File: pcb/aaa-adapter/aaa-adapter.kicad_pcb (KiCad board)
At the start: 2 copper layers, 51.5 x 38 mm, 2 parts

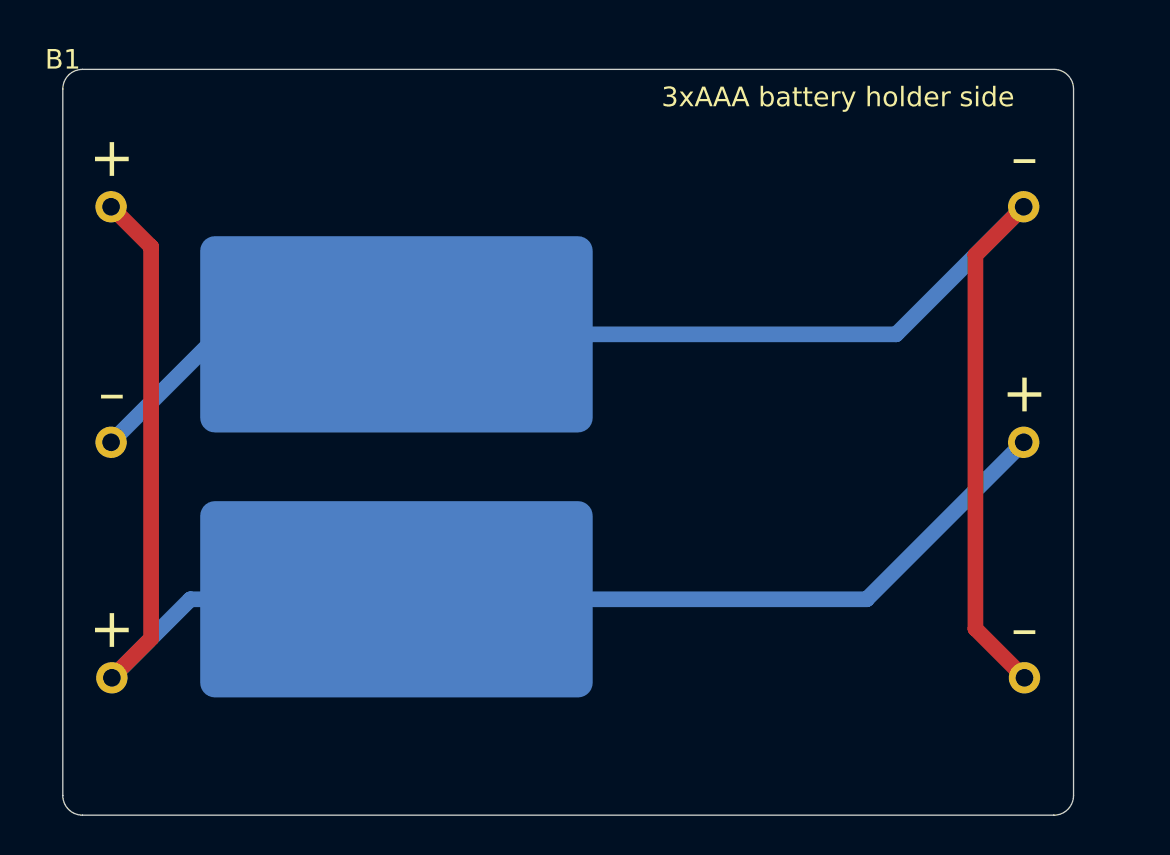
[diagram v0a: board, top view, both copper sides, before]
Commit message: production
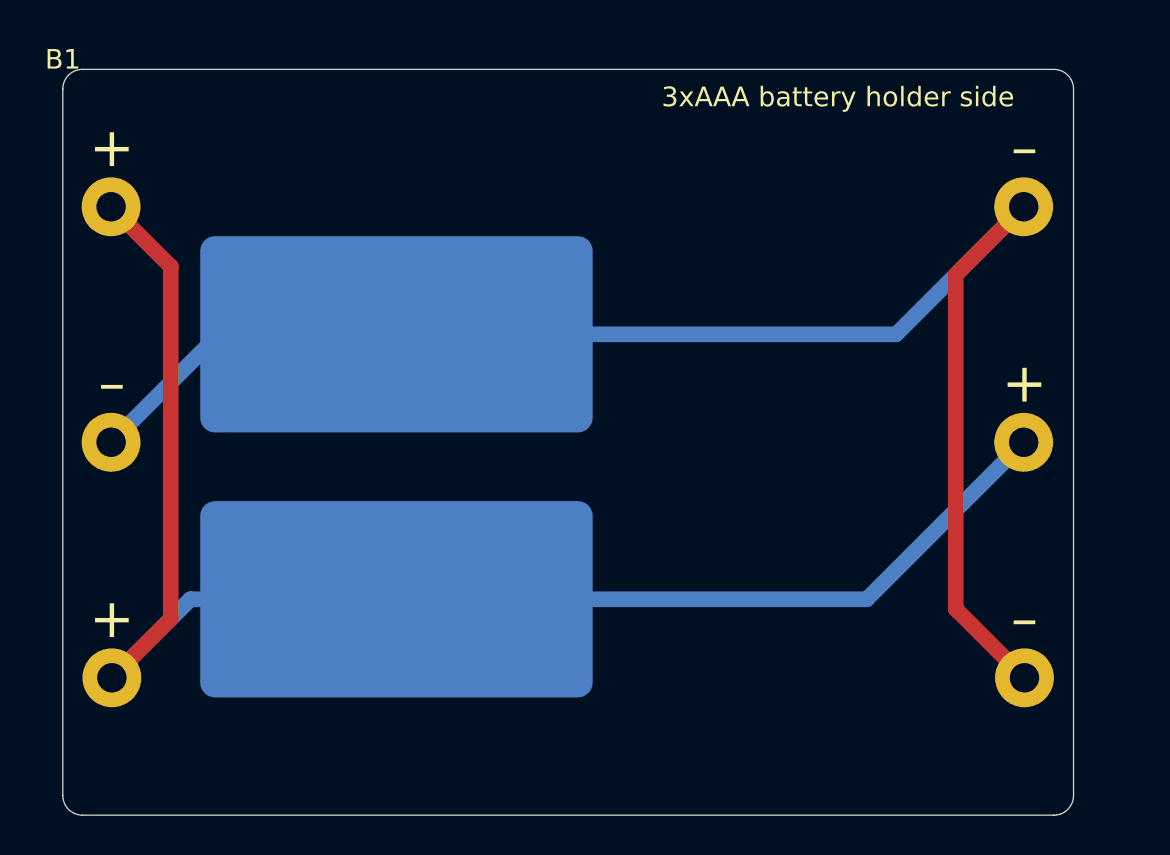
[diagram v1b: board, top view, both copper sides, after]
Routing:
- net /V-: track 77.5 -> 78.4 mm
- net /V+: track 77.1 -> 77.9 mm
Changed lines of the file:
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@@
 		(pad "1" thru_hole circle
 			(at 2.46 7)
-			(size 1.6 1.6)
-			(drill 0.9)
+			(size 3 3)
+			(drill 1.5)
 			(layers "*.Cu" "*.Mask")
 			(remove_unused_layers no)
@@
 		(pad "2" thru_hole circle
 			(at 2.46 19)
-			(size 1.6 1.6)
-			(drill 0.9)
+			(size 3 3)
+			(drill 1.5)
 			(layers "*.Cu" "*.Mask")
 			(remove_unused_layers no)
@@
 		(pad "3" thru_hole circle
 			(at 2.5 31)
-			(size 1.6 1.6)
-			(drill 0.9)
+			(size 3 3)
+			(drill 1.5)
 			(layers "*.Cu" "*.Mask")
 			(remove_unused_layers no)
@@
 		(pad "4" thru_hole circle
 			(at 49 31)
-			(size 1.6 1.6)
-			(drill 0.9)
+			(size 3 3)
+			(drill 1.5)
 			(layers "*.Cu" "*.Mask")
 			(remove_unused_layers no)
@@
 		(pad "5" thru_hole circle
 			(at 48.96 19)
-			(size 1.6 1.6)
-			(drill 0.9)
+			(size 3 3)
+			(drill 1.5)
 			(layers "*.Cu" "*.Mask")
 			(remove_unused_layers no)
@@
 		(pad "6" thru_hole circle
 			(at 48.96 7)
-			(size 1.6 1.6)
-			(drill 0.9)
+			(size 3 3)
+			(drill 1.5)
 			(layers "*.Cu" "*.Mask")
 			(remove_unused_layers no)
@@
 	)
 	(gr_text "–"
-		(at 17.5 31.5 0)
+		(at 17.5 31 0)
 		(layer "F.SilkS")
 		(effects
@@
 	)
 	(gr_text "–"
-		(at 64 19.5 0)
+		(at 64 19 0)
 		(layer "F.SilkS")
 		(effects
@@
 	)
 	(gr_text "+"
-		(at 64 31.5 0)
+		(at 64 31 0)
 		(layer "F.SilkS")
 		(effects
@@
 	)
 	(gr_text "+"
-		(at 17.5 19.5 0)
+		(at 17.5 19 0)
 		(layer "F.SilkS")
 		(effects
@@
 	)
 	(gr_text "+"
-		(at 17.5 43.5 0)
+		(at 17.5 43 0)
 		(layer "F.SilkS")
 		(effects
@@
 	)
 	(gr_text "–"
-		(at 64 43.5 0)
-		(layer "F.SilkS")
-		(effects
-			(font
-				(size 2 2)
-				(thickness 0.25)
-			)
-		)
-	)
-	(segment
-		(start 61.5 43.5)
+		(at 64 43 0)
+		(layer "F.SilkS")
+		(effects
+			(font
+				(size 2 2)
+				(thickness 0.25)
+			)
+		)
+	)
+	(segment
+		(start 60.5 42.5)
 		(end 64 46)
 		(width 0.8)
@@
 	)
 	(segment
-		(start 61.5 24.46)
-		(end 61.5 43.5)
+		(start 63.96 22)
+		(end 60.5 25.46)
 		(width 0.8)
 		(layer "F.Cu")
@@
 	)
 	(segment
-		(start 63.96 22)
-		(end 61.5 24.46)
+		(start 60.5 25.46)
+		(end 60.5 42.5)
 		(width 0.8)
 		(layer "F.Cu")
@@
 	)
 	(segment
-		(start 19.5 44)
-		(end 17.5 46)
+		(start 20.5 25.04)
+		(end 20.5 43)
 		(width 0.8)
 		(layer "F.Cu")
@@
 	(segment
 		(start 17.46 22)
-		(end 19.5 24.04)
+		(end 20.5 25.04)
 		(width 0.8)
 		(layer "F.Cu")
@@
 	)
 	(segment
-		(start 19.5 24.04)
-		(end 19.5 44)
+		(start 20.5 43)
+		(end 17.5 46)
 		(width 0.8)
 		(layer "F.Cu")
